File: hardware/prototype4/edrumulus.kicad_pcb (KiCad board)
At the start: 2 copper layers, 65 x 56.5 mm, 67 parts, among them J1 Trigger Connector, J2 Raspberry Pi GPIO pins, U1 ESP32-DEVKIT-V1

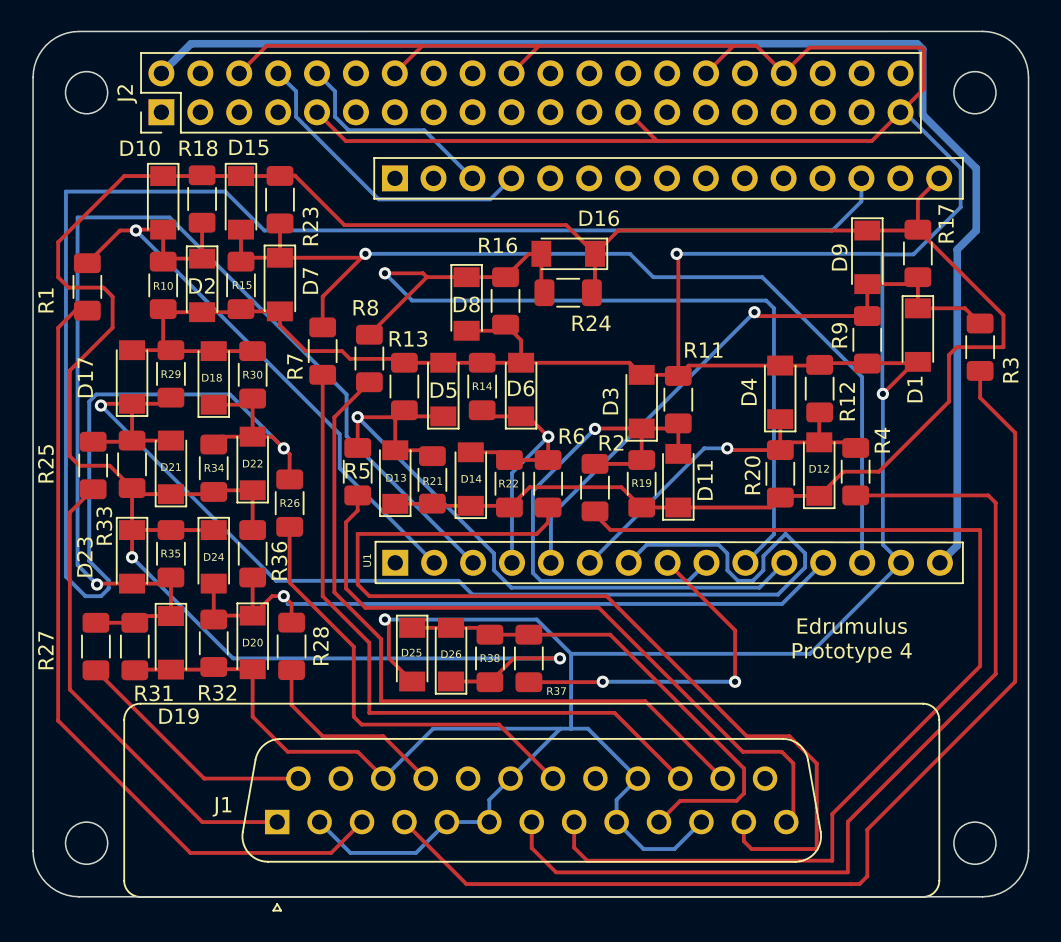
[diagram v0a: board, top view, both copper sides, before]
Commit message: some more optimizations for prototype 4
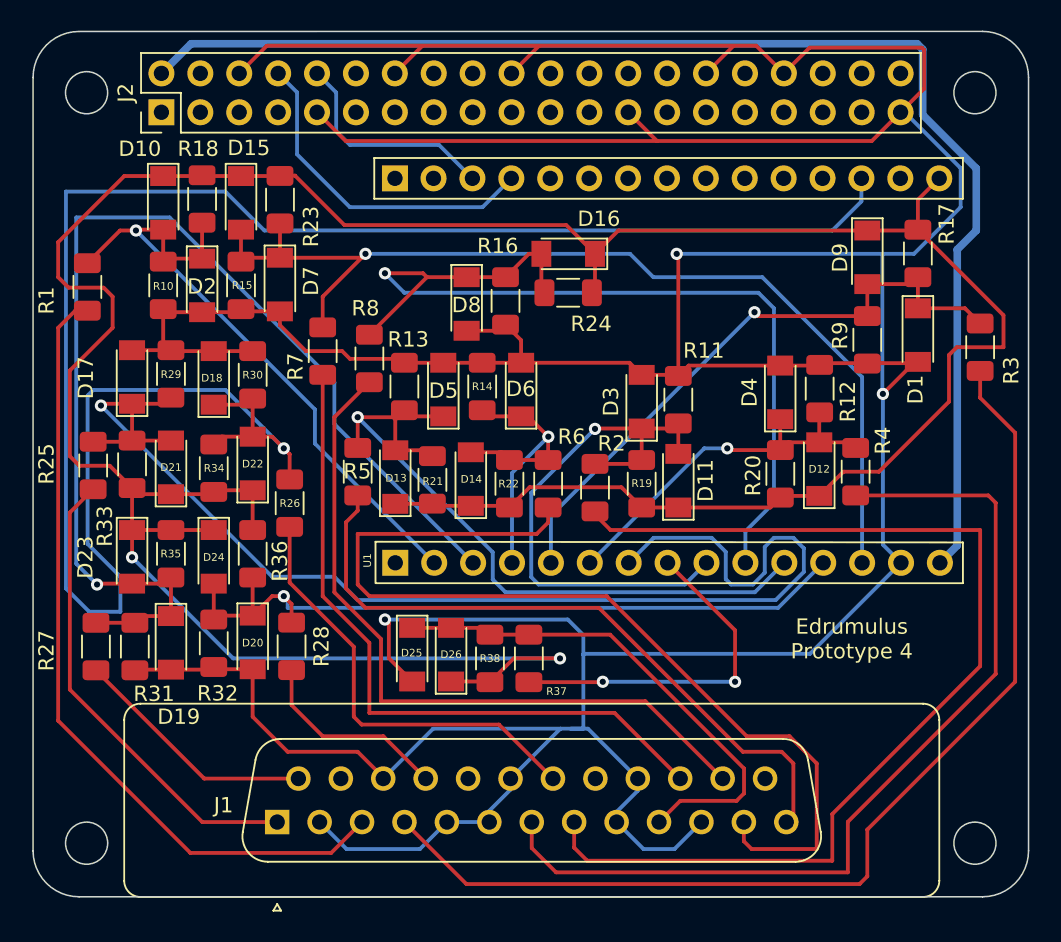
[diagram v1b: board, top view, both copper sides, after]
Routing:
- net GPIO15: track 123.5 -> 127.4 mm
- net ESP-UART0-RX: track 20.2 -> 22.0 mm
- net GPIO33: track 81.2 -> 82.9 mm
- net CRASH1-SLEEVE: track 348.8 -> 350.1 mm
- net GPIO14: track 47.2 -> 47.8 mm
- net GPIO26: track 35.9 -> 36.4 mm
- net ESP-UART0-TX: track 14.0 -> 14.5 mm

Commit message: added filler
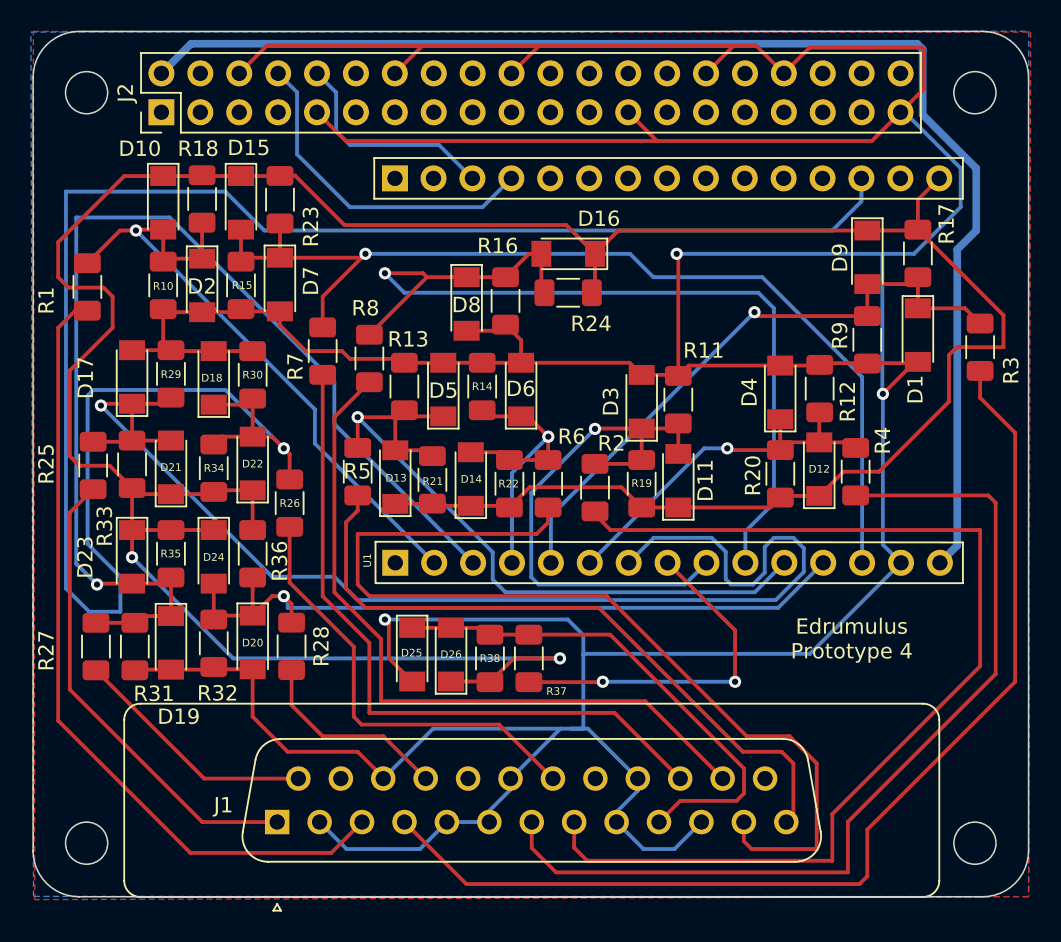
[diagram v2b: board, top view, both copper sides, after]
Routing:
- added copper zone on B.Cu, net CRASH1-SLEEVE
- added copper zone on F.Cu, net CRASH1-SLEEVE
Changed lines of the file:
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@@
   (via (at 143.764 115.57) (size 0.8) (drill 0.4) (layers "F.Cu" "B.Cu") (net 64))
   (segment (start 143.764 115.57) (end 152.4 115.57) (width 0.25) (layer "B.Cu") (net 64))
+  (zone (net 1) (net_name "CRASH1-SLEEVE") (layer "F.Cu") (hatch edge 0.508)
+    (connect_pads (clearance 0.508))
+    (min_thickness 0.254) (filled_areas_thickness no)
+    (fill yes (thermal_gap 0.508) (thermal_bridge_width 0.508))
+    (polygon
+      (pts
+        (xy 171.561542 129.601205)
+        (xy 106.68 129.794)
+        (xy 106.584157 73.107062)
+        (xy 171.704 73.152)
+      )
+    )
+  )
+  (zone (net 1) (net_name "CRASH1-SLEEVE") (layer "B.Cu") (hatch edge 0.508)
+    (connect_pads (clearance 0.508))
+    (min_thickness 0.254) (filled_areas_thickness no)
+    (fill yes (thermal_gap 0.508) (thermal_bridge_width 0.508))
+    (polygon
+      (pts
+        (xy 171.573414 129.597233)
+        (xy 106.595381 129.584665)
+        (xy 106.426 73.152)
+        (xy 171.580429 73.096443)
+      )
+    )
+  )
   (group "" locked (id 1d468920-09d8-44ff-9425-46d8affb1930)
     (members
